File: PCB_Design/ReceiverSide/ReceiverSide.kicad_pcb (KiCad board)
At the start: 2 copper layers, 17 parts, among them J1 Conn_01x02_Pin

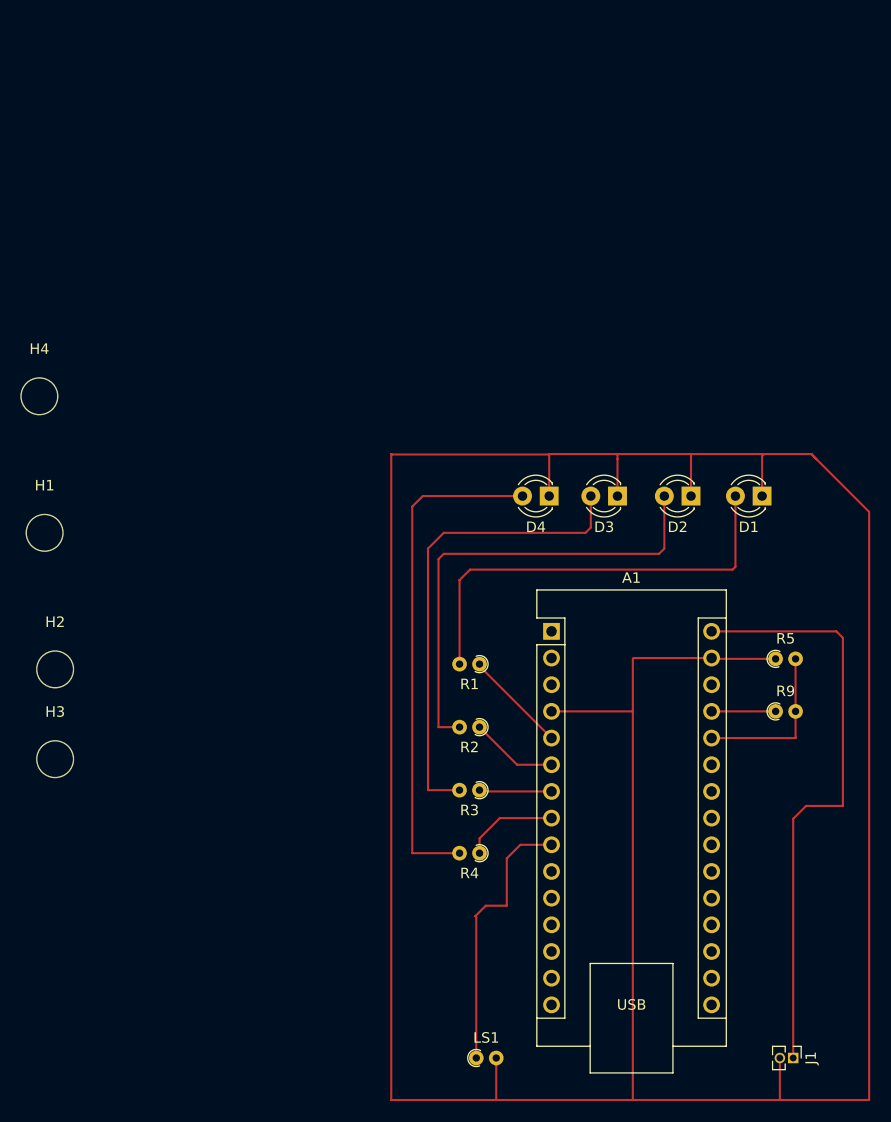
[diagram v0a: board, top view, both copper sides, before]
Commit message: fix
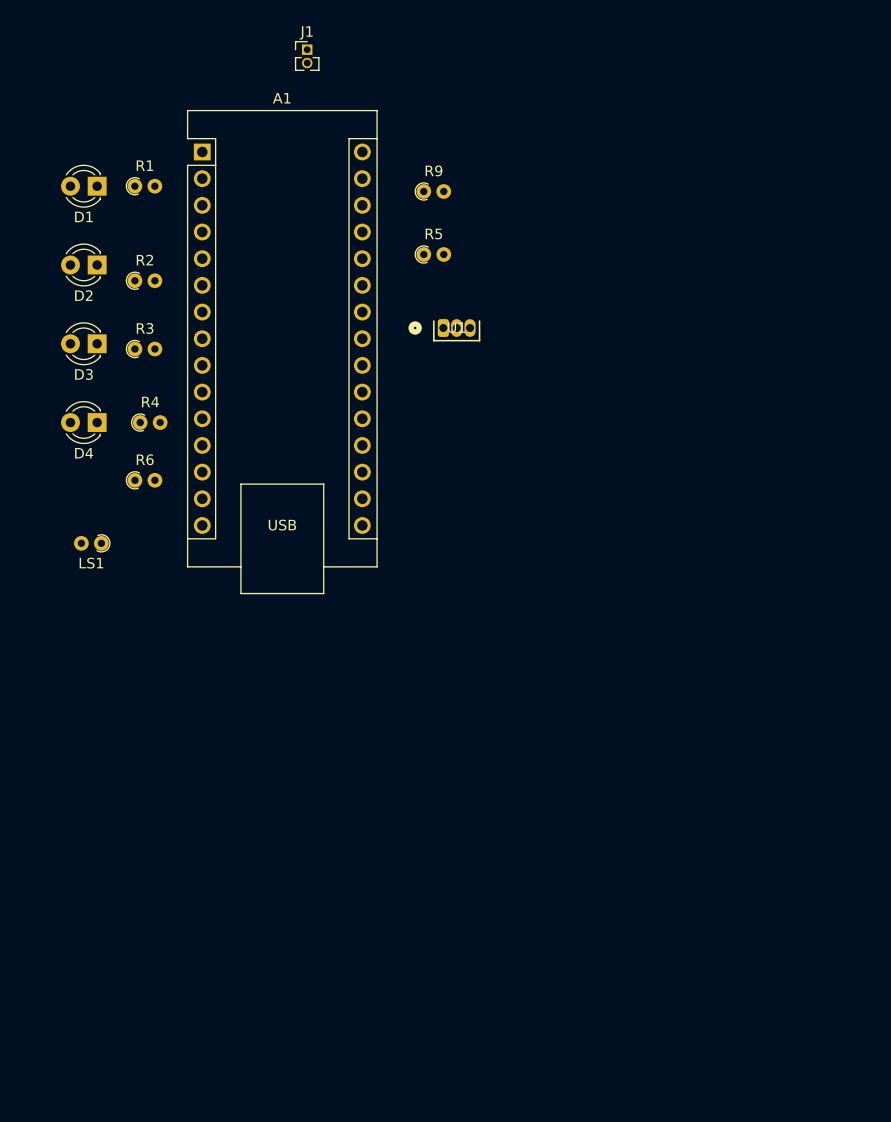
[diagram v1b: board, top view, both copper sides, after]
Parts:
- removed H1, H2, H3, H4: MountingHole, MountingHole:MountingHole_3.5mm
- added R6: R, Resistor_THT:R_Axial_DIN0204_L3.6mm_D1.6mm_P1.90mm_Vertical, F.Cu at (117.6, 87.0)
- added U1: DRV5053CAQLPGM, Halleffect:LPG3_TEX, F.Cu at (147.0, 72.5)
- moved J1 106.6 mm to (134.0, 46.0), turned to 0 degrees
- moved D1 69.8 mm to (114.0, 59.0)
- moved D2 60.7 mm to (114.0, 66.5)
- moved LS1 60.6 mm to (114.4, 93.0), turned to 180 degrees
- moved R9 59.8 mm to (145.1, 59.5)
- moved A1 56.5 mm to (124.0, 55.7)
- moved R1 56.1 mm to (117.6, 59.0), turned to 0 degrees
- moved R2 53.7 mm to (117.6, 68.0), turned to 0 degrees
- moved R3 53.3 mm to (117.6, 74.5), turned to 0 degrees
- moved R4 52.2 mm to (118.1, 81.5), turned to 0 degrees
- moved D3 51.6 mm to (114.0, 74.0)
- moved R5 51.0 mm to (145.1, 65.5)
- moved D4 43.6 mm to (114.0, 81.5)
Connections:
- D1 pad 1: GND -> /LEDa
- D1 pad 2: /LEDa -> GND
- D2 pad 1: GND -> /LEDb
- D2 pad 2: /LEDb -> GND
- D3 pad 1: GND -> /LEDc
- D3 pad 2: /LEDc -> GND
- D4 pad 1: GND -> /LEDd
- D4 pad 2: /LEDd -> GND
- LS1 pad 1: /D6 -> /Speaker
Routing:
- net GND: track 299.1 -> 0.00 mm
- net Net-(A1-VIN): track 56.8 -> 0.00 mm
- net /LEDd: track 48.4 -> 0.00 mm
- net /LEDc: track 45.3 -> 0.00 mm
- net /LEDb: track 44.9 -> 0.00 mm
- net /LEDa: track 41.5 -> 0.00 mm
- net /D6: track 26.3 -> 0.00 mm
- net /Photores: track 16.0 -> 0.00 mm
- net /LED1: track 9.88 -> 0.00 mm
- net /LED4: track 9.06 -> 0.00 mm
- net /LED2: track 8.34 -> 0.00 mm
- net /LED3: track 6.91 -> 0.00 mm
- net +5V: track 6.09 -> 0.00 mm

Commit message: transmitter pcb
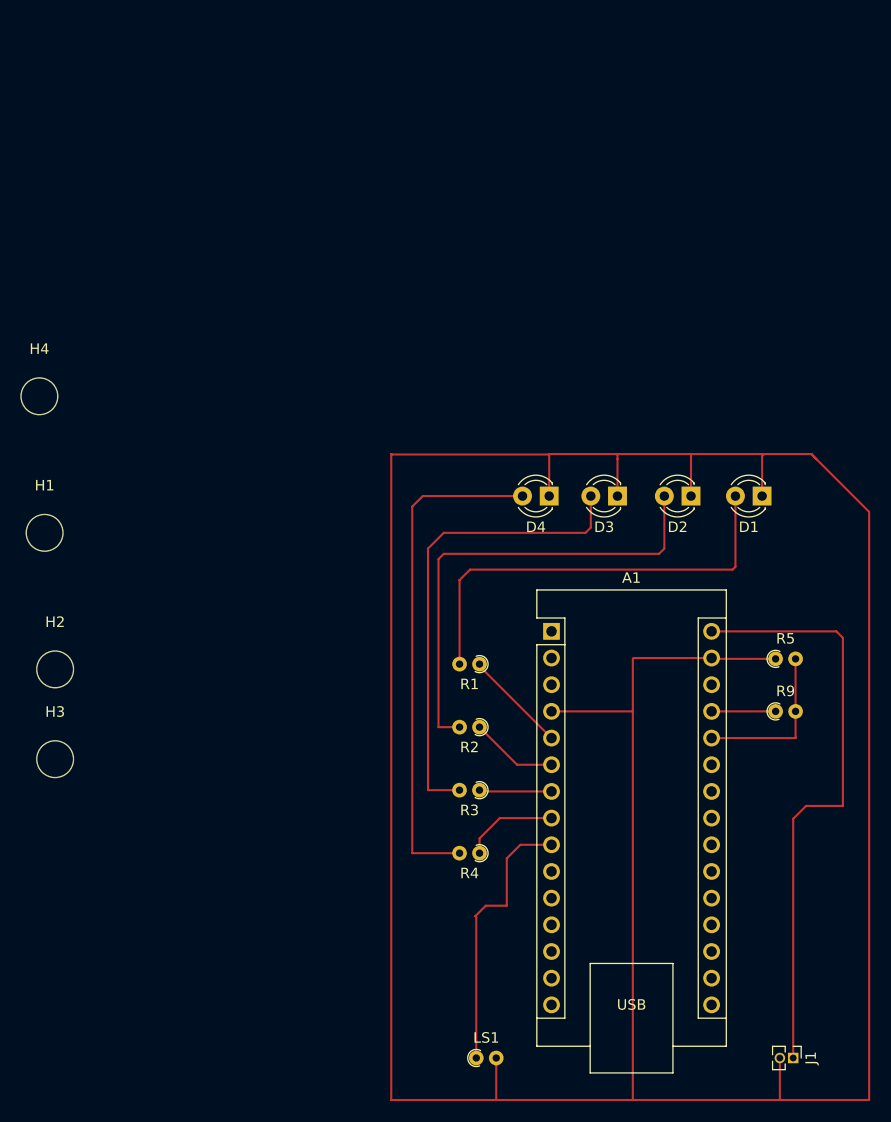
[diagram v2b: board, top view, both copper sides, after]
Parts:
- removed R6: R, Resistor_THT:R_Axial_DIN0204_L3.6mm_D1.6mm_P1.90mm_Vertical
- removed U1: DRV5053CAQLPGM, Halleffect:LPG3_TEX
- added H1: MountingHole, MountingHole:MountingHole_3.5mm, F.Cu at (109.0, 92.0)
- added H2: MountingHole, MountingHole:MountingHole_3.5mm, F.Cu at (110.0, 105.0)
- added H3: MountingHole, MountingHole:MountingHole_3.5mm, F.Cu at (110.0, 113.5)
- added H4: MountingHole, MountingHole:MountingHole_3.5mm, F.Cu at (108.5, 79.0)
- moved J1 106.6 mm to (180.3, 142.0), turned to -90 degrees
- moved D1 69.8 mm to (177.3, 88.5)
- moved D2 60.7 mm to (170.5, 88.5)
- moved LS1 60.6 mm to (150.1, 142.0), turned to 0 degrees
- moved R9 59.8 mm to (178.6, 109.0)
- moved A1 56.5 mm to (157.3, 101.4)
- moved R1 56.1 mm to (150.4, 104.5), turned to 180 degrees
- moved R2 53.7 mm to (150.4, 110.5), turned to 180 degrees
- moved R3 53.3 mm to (150.4, 116.5), turned to 180 degrees
- moved R4 52.2 mm to (150.4, 122.5), turned to 180 degrees
- moved D3 51.6 mm to (163.5, 88.5)
- moved R5 51.0 mm to (178.6, 104.0)
- moved D4 43.6 mm to (157.0, 88.5)
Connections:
- D1 pad 1: /LEDa -> GND
- D1 pad 2: GND -> /LEDa
- D2 pad 1: /LEDb -> GND
- D2 pad 2: GND -> /LEDb
- D3 pad 1: /LEDc -> GND
- D3 pad 2: GND -> /LEDc
- D4 pad 1: /LEDd -> GND
- D4 pad 2: GND -> /LEDd
- LS1 pad 1: /Speaker -> /D6
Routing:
- net GND: track 0.00 -> 299.1 mm
- net Net-(A1-VIN): track 0.00 -> 56.8 mm
- net /LEDd: track 0.00 -> 48.4 mm
- net /LEDc: track 0.00 -> 45.3 mm
- net /LEDb: track 0.00 -> 44.9 mm
- net /LEDa: track 0.00 -> 41.5 mm
- net /D6: track 0.00 -> 26.3 mm
- net /Photores: track 0.00 -> 16.0 mm
- net /LED1: track 0.00 -> 9.88 mm
- net /LED4: track 0.00 -> 9.06 mm
- net /LED2: track 0.00 -> 8.34 mm
- net /LED3: track 0.00 -> 6.91 mm
- net +5V: track 0.00 -> 6.09 mm
